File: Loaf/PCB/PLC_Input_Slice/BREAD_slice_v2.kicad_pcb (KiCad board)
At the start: 2 copper layers, 100 x 70.6 mm, 34 parts, among them J1 10018783-10200TLF, J3 DB25_Socket, U1 MCP4922-EP, U2 MCP4922-EP, U3 MCP4922-EP, U4 MCP4922-EP, U5 MCP3208, U6 MCP2561-E-P, U7 MCP2515-xSO, Y1 16MHZ Crystal

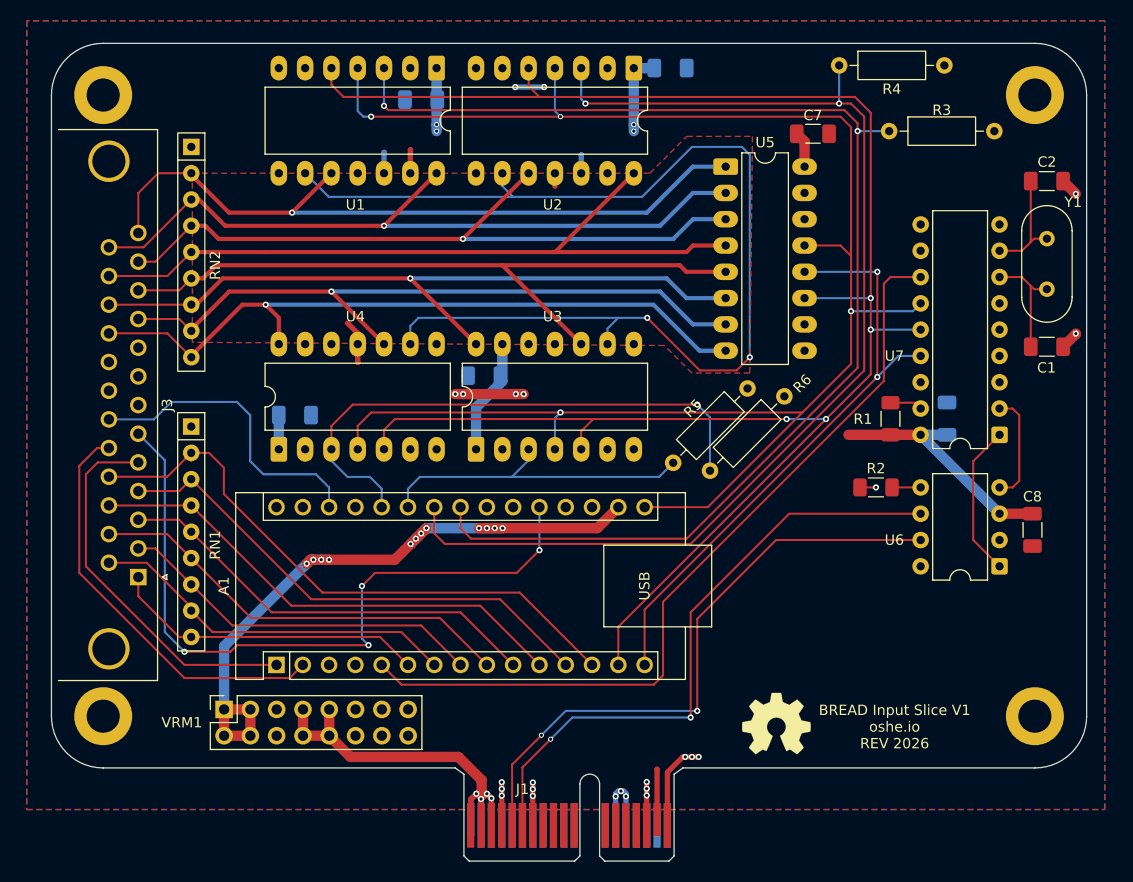
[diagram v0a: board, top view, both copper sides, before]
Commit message: Add files via upload
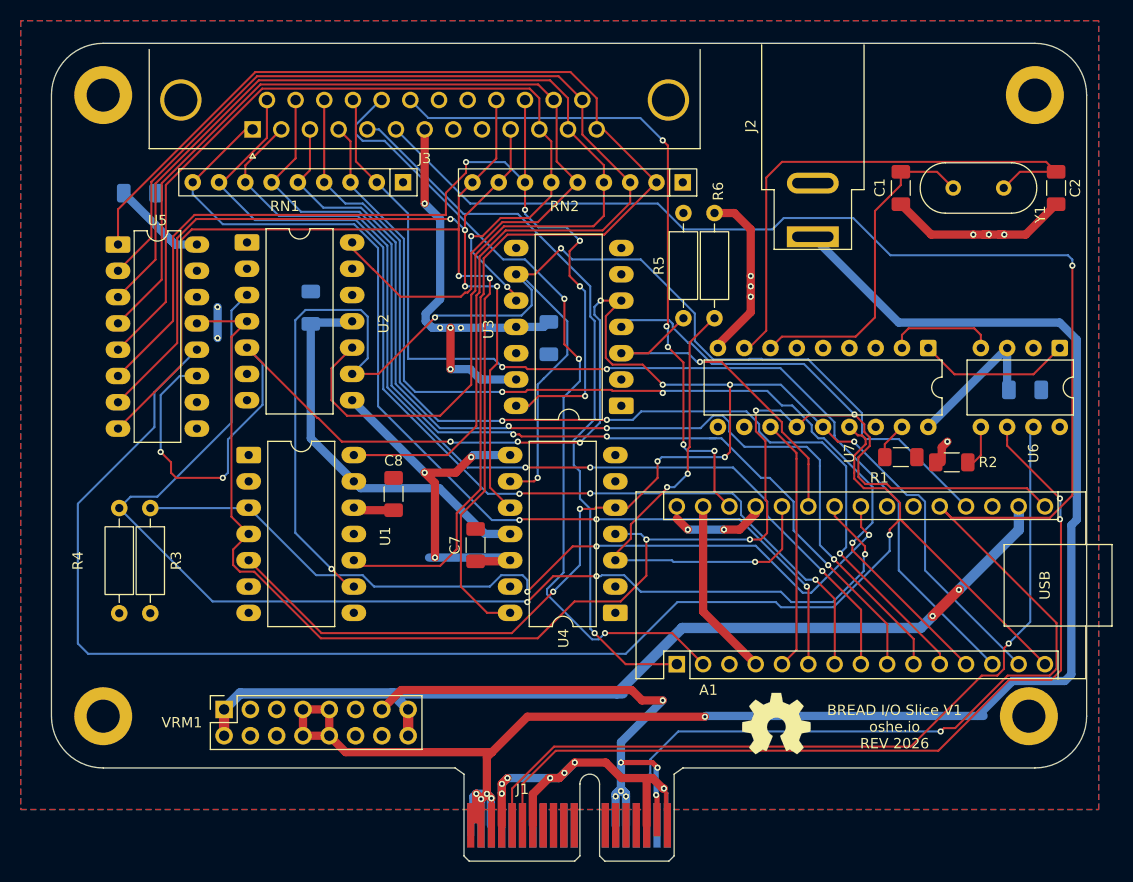
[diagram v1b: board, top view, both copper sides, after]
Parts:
- removed C9: 0.47uF, Capacitor_SMD:C_1206_3216Metric_Pad1.33x1.80mm_HandSolder
- added J2: Barrel Jack, Connector_BarrelJack:BarrelJack_SwitchcraftConxall_RAPC10U_Horizontal, F.Cu at (175.0, 74.2)
- moved R4 81.6 mm to (108.0, 100.4), turned to -90 degrees
- moved R3 80.1 mm to (111.0, 100.4), turned to -90 degrees
- moved C3 64.7 mm to (195.5, 89.0), turned to 180 degrees
- moved C8 61.8 mm to (134.5, 99.1)
- moved U5 59.2 mm to (107.9, 75.0)
- moved C4 52.7 mm to (110.0, 70.0)
- moved C7 51.4 mm to (142.4, 104.0), turned to 90 degrees
- moved RN2 47.6 mm to (162.4, 69.0), turned to 180 degrees
- moved J3 44.6 mm to (120.9, 63.8), turned to 180 degrees
- moved U1 41.6 mm to (120.5, 95.3), turned to 0 degrees
- moved U2 41.0 mm to (120.3, 74.8), turned to 0 degrees
- moved A1 38.7 mm to (161.9, 115.5)
- moved U4 36.1 mm to (155.9, 110.5), turned to 180 degrees
- moved RN1 31.2 mm to (135.4, 69.0), turned to 180 degrees
- moved U6 21.9 mm to (198.8, 85.0), turned to -90 degrees
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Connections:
- A1 pad 19: /SHDNTRIG -> /SHDN
- J1 pad A16: /EstpCh1 -> /ESTOP
- VRM1 pad 15: +5V -> +3.3V
- VRM1 pad 16: +5V -> +3.3V
- VRM1 pad 3: +3.3V -> +5V
- VRM1 pad 4: +3.3V -> +5V
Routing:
- net +12V: track 53.0 -> 172.3 mm, vias 4 -> 5
- net /ESTOP: track 69.7 -> 178.1 mm, vias 4 -> 2
- net GND: track 36.8 -> 141.9 mm, vias 19 -> 17
- net +5V: track 78.5 -> 174.8 mm, vias 9 -> 16
- net /MISO: track 59.3 -> 154.2 mm, vias 2 -> 1
- net /DIO0: track 30.9 -> 100.7 mm, vias 0 -> 3
- net /DIO1: track 35.7 -> 101.4 mm, vias 0 -> 3
- net /DIO2: track 35.8 -> 97.2 mm, vias 0 -> 3
- net /DIO3: track 41.8 -> 100.2 mm, vias 0 -> 3
- net /DIO4: track 42.0 -> 100.3 mm, vias 0 -> 3
- net /AIO0: track 70.3 -> 126.8 mm, vias 1 -> 0
- net /DIO5: track 48.0 -> 102.3 mm, vias 0 -> 3
- net /INT: track 78.8 -> 24.5 mm
- net /DIO6: track 49.2 -> 99.6 mm, vias 0 -> 3
- net /AIO2: track 68.5 -> 117.9 mm, vias 1 -> 0
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- removed copper zone on F.Cu, net GND
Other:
- board text added: "BREAD I/O Slice V1 oshe.io REV 2026"
- board text removed: "BREAD Input Slice V1 oshe.io REV 2026"
